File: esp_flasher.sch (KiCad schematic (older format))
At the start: 29 parts, among them J1 USB_B_Micro, J2 Conn_01x06, J3 boot btn, J4 en btn, Q1 S8050, Q2 S8050, U1 ZLDO1117QG33TA_SOT223, U2 CP2102N-A01-GQFN28

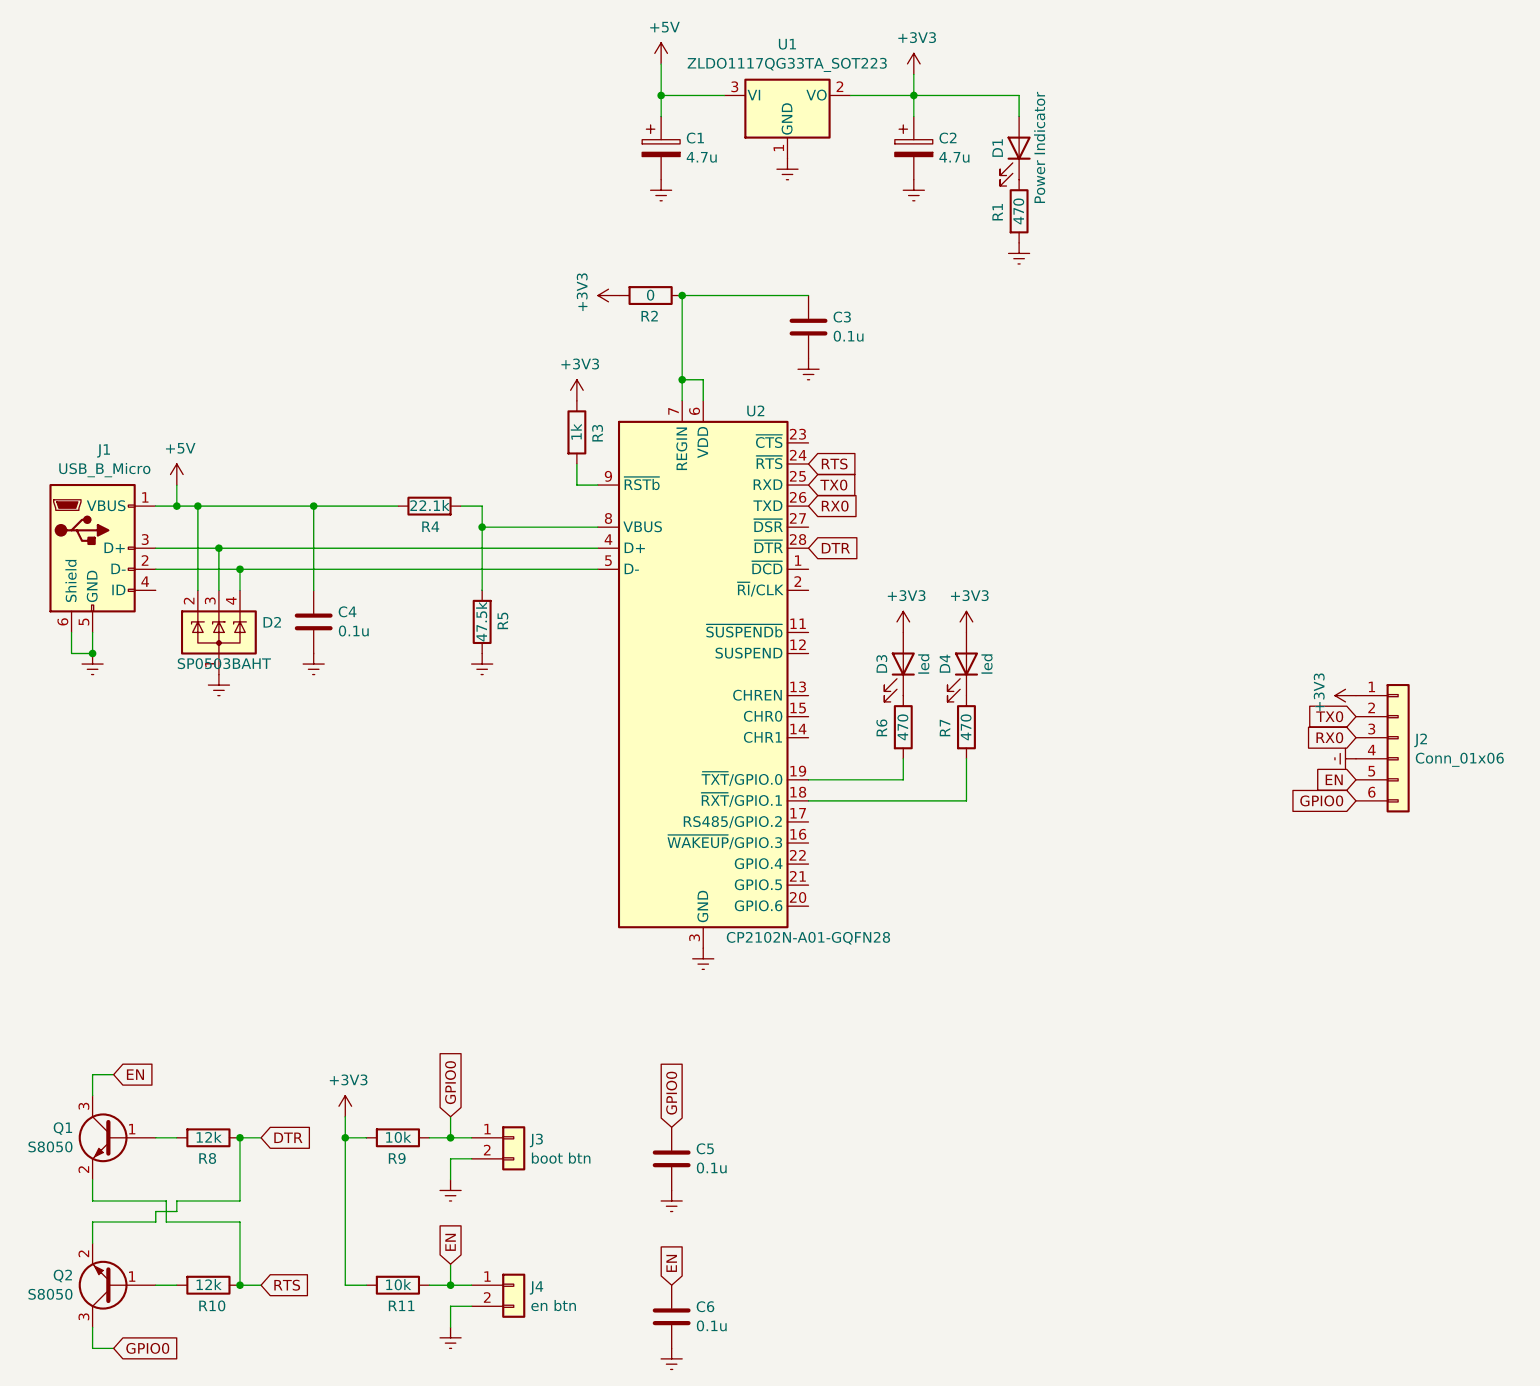
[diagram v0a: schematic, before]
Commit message: 2021-07-20 2
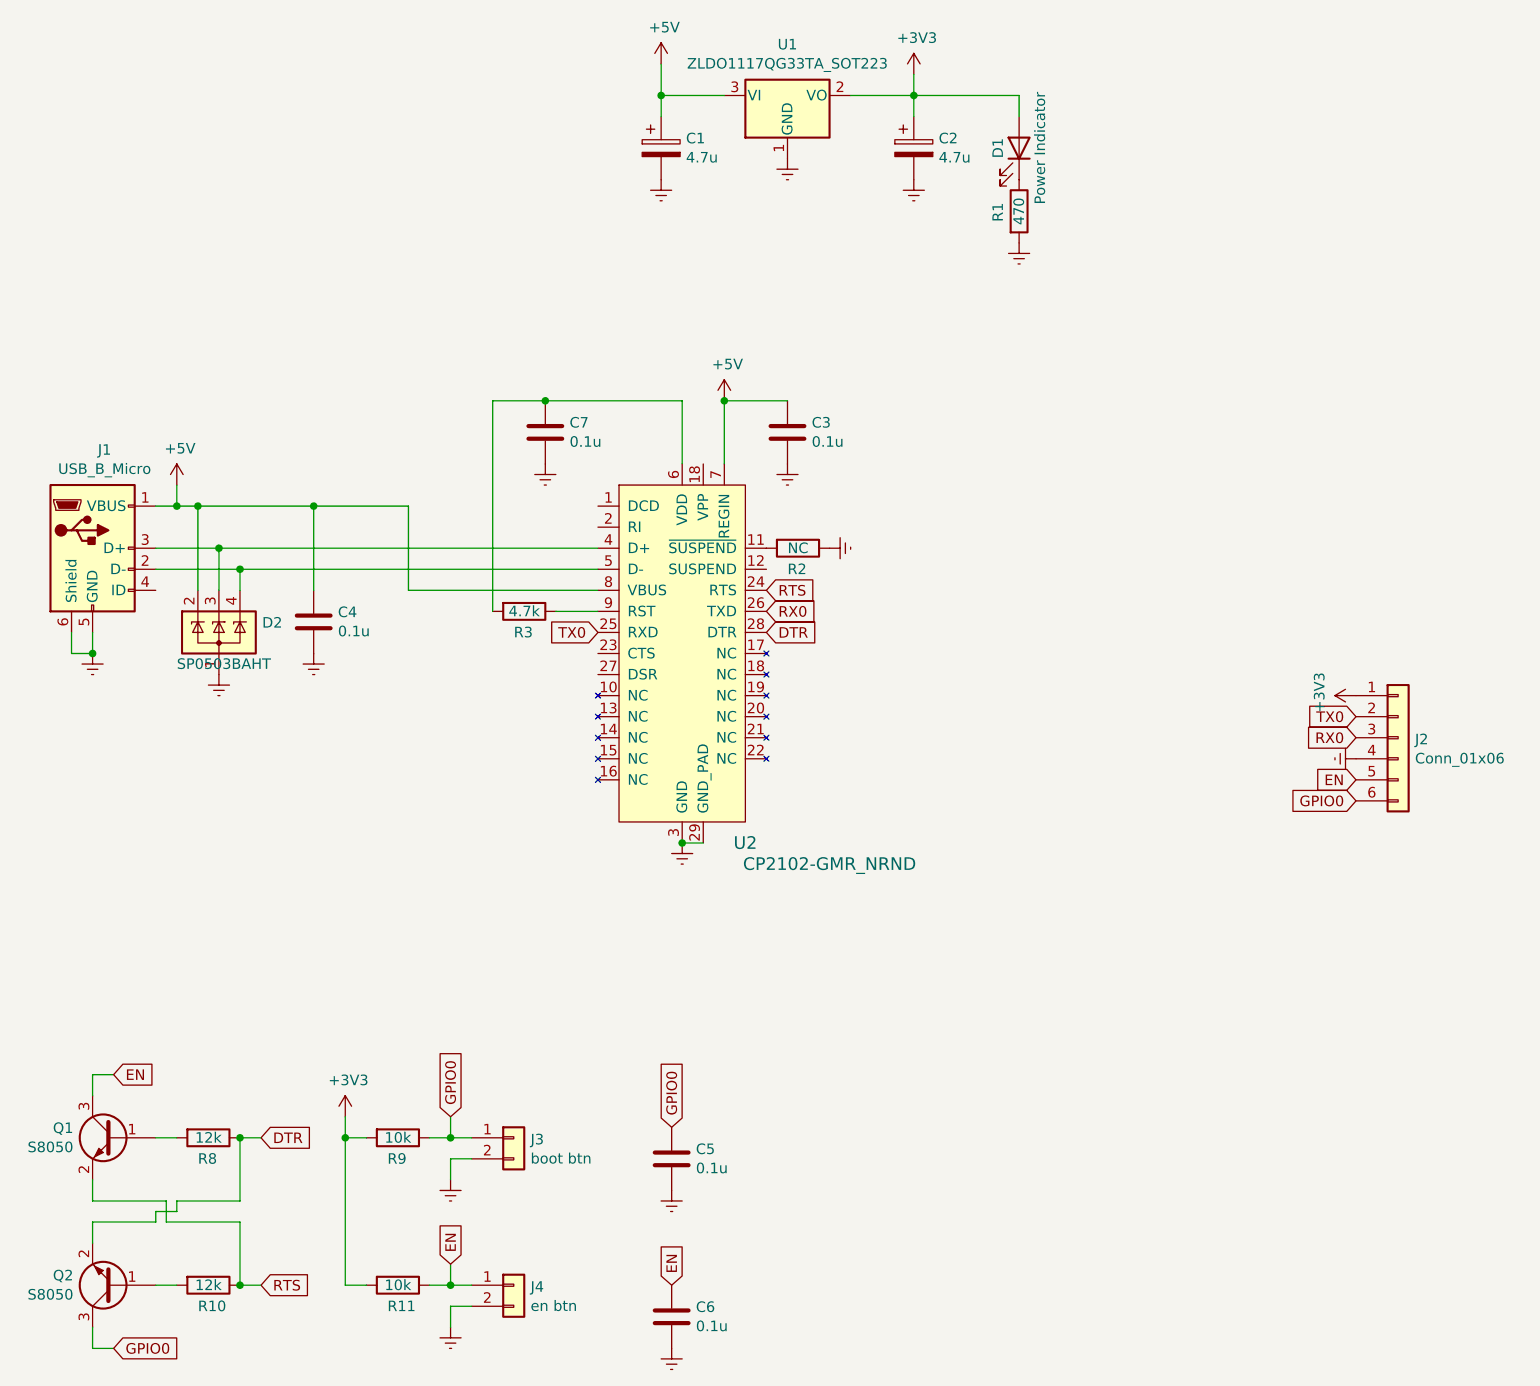
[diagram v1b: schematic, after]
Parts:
- removed D3, D4: led, LED_SMD:LED_0805_2012Metric_Pad1.15x1.40mm_HandSolder, symbol Device:LED
- removed R4: 22.1k, Resistor_SMD:R_0603_1608Metric_Pad0.98x0.95mm_HandSolder, symbol Device:R
- removed R5: 47.5k, Resistor_SMD:R_0603_1608Metric_Pad0.98x0.95mm_HandSolder, symbol Device:R
- removed R6, R7: 470, Resistor_SMD:R_0603_1608Metric_Pad0.98x0.95mm_HandSolder, symbol Device:R
- removed U2: CP2102N-A01-GQFN28, Package_DFN_QFN:QFN-28-1EP_5x5mm_P0.5mm_EP3.35x3.35mm, symbol Interface_USB:CP2102N-A01-GQFN28
- added C7: 0.1u, Capacitor_SMD:C_0603_1608Metric_Pad1.08x0.95mm_HandSolder, symbol Device:C
- added U2: CP2102-GMR_NRND, digikey-footprints:VFQFN-28-1EP_5x5mm, symbol dk_Interface-Controllers:CP2102-GMR_NRND
- J1: footprint Connector_USB:USB_Micro-B_GCT_USB3076-30-A -> Connector_USB:USB_Micro-AB_Molex_47590-0001
- R2: value 0 -> NC
- R3: value 1k -> 4.7k
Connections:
- net +3V3: no longer R2.2, R3.1
- net +5V: now also C3.1, U2.7 (REGIN), U2.8 (VBUS)
- net DTR: now also U2.28 (DTR)
- net Earth: now also R2.1, C7.2, U2.29 (GND_PAD), U2.3 (GND)
- net RTS: now also U2.24 (RTS)
- net RX0: now also U2.26 (TXD)
- net TX0: now also U2.25 (RXD)
- net at D2.4 (K), J1.2 (D-): now also U2.5 (D-)
- net at D2.3 (K), J1.3 (D+): now also U2.4 (D+)
- net at R3.2: now also C7.1, U2.6 (VDD)
- new net: R3.1, U2.9 (RST)
- new net: R2.2, U2.11 (~SUSPEND)
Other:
- moved on the sheet: C3, R2, R3
